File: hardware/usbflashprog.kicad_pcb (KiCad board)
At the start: 2 copper layers, 211 x 122 mm, 121 parts, among them J2 Parallel Adapter, J3 Serial Adapter, Q1 BC547, Q10 BC557, Q11 BC557, Q12 BC547, Q13 BC547, Q14 BC547, Q15 BC547, Q16 BC547, Q2 BC327, Q3 BC327, Q4 BC327, Q5 TIP120, Q6 BC327, Q7 BC557, Q8 BC557, Q9 BC557, U1 MT3608 Module, U10 74HC595, U11 74HC165, U12 74HC165, U2 74LS06N, U3 Pico, U4 74HC595, U5 74HC595, U6 74HC595, U7 74HC595, U8 74LS06N, U9 74HC595

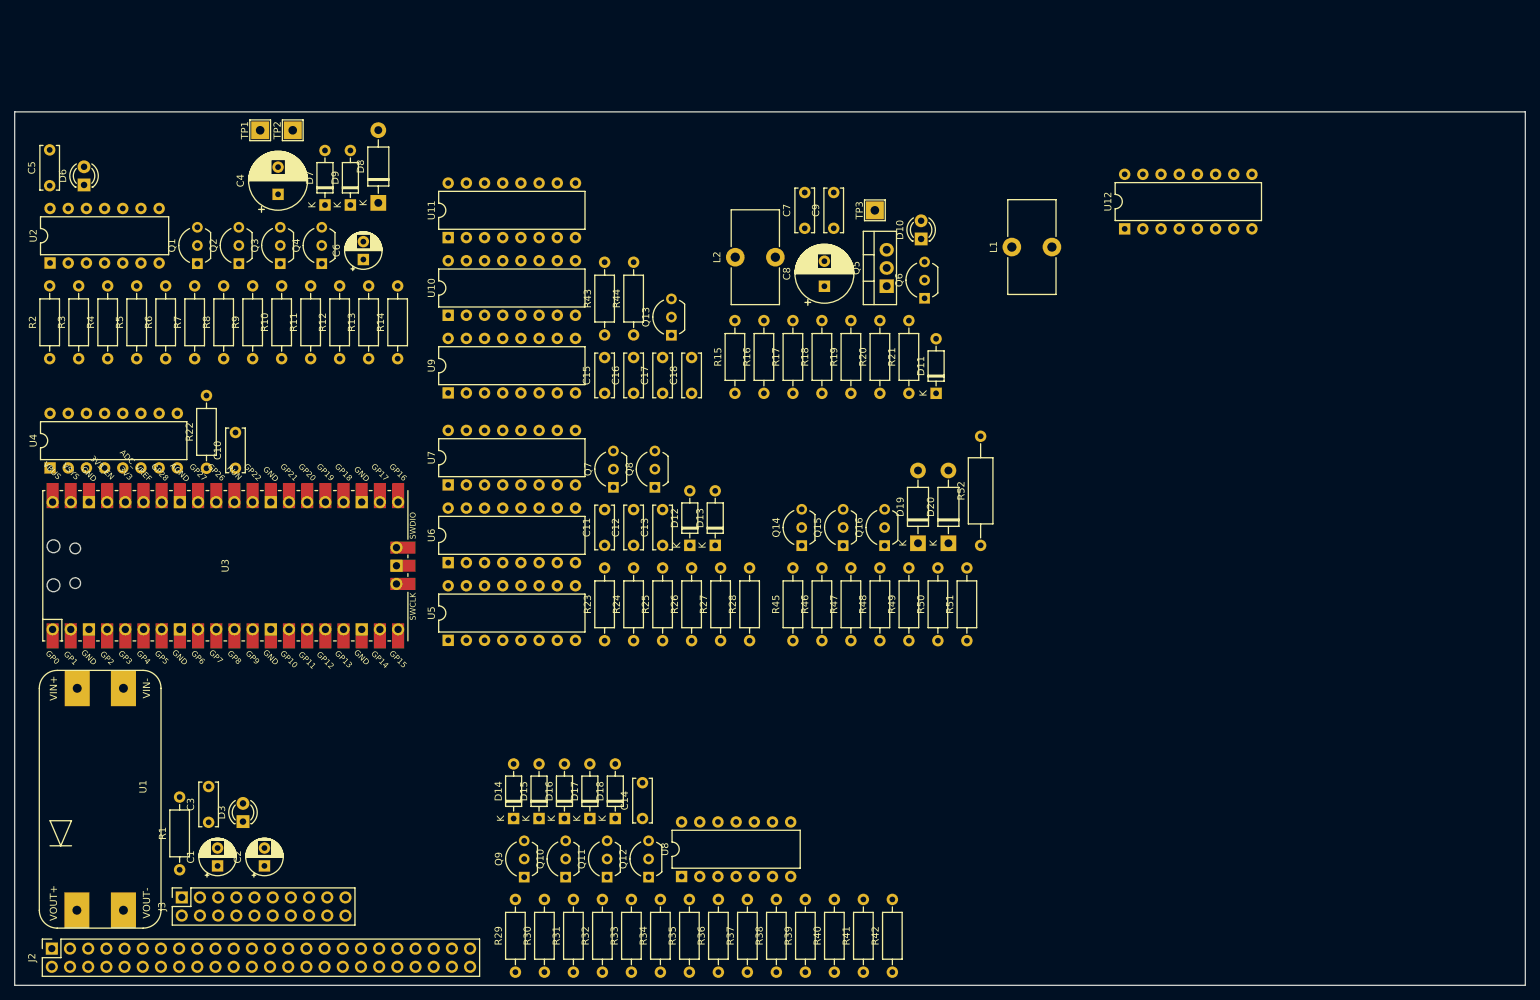
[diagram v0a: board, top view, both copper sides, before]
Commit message: 0.3.rev.A. Created new main pcb
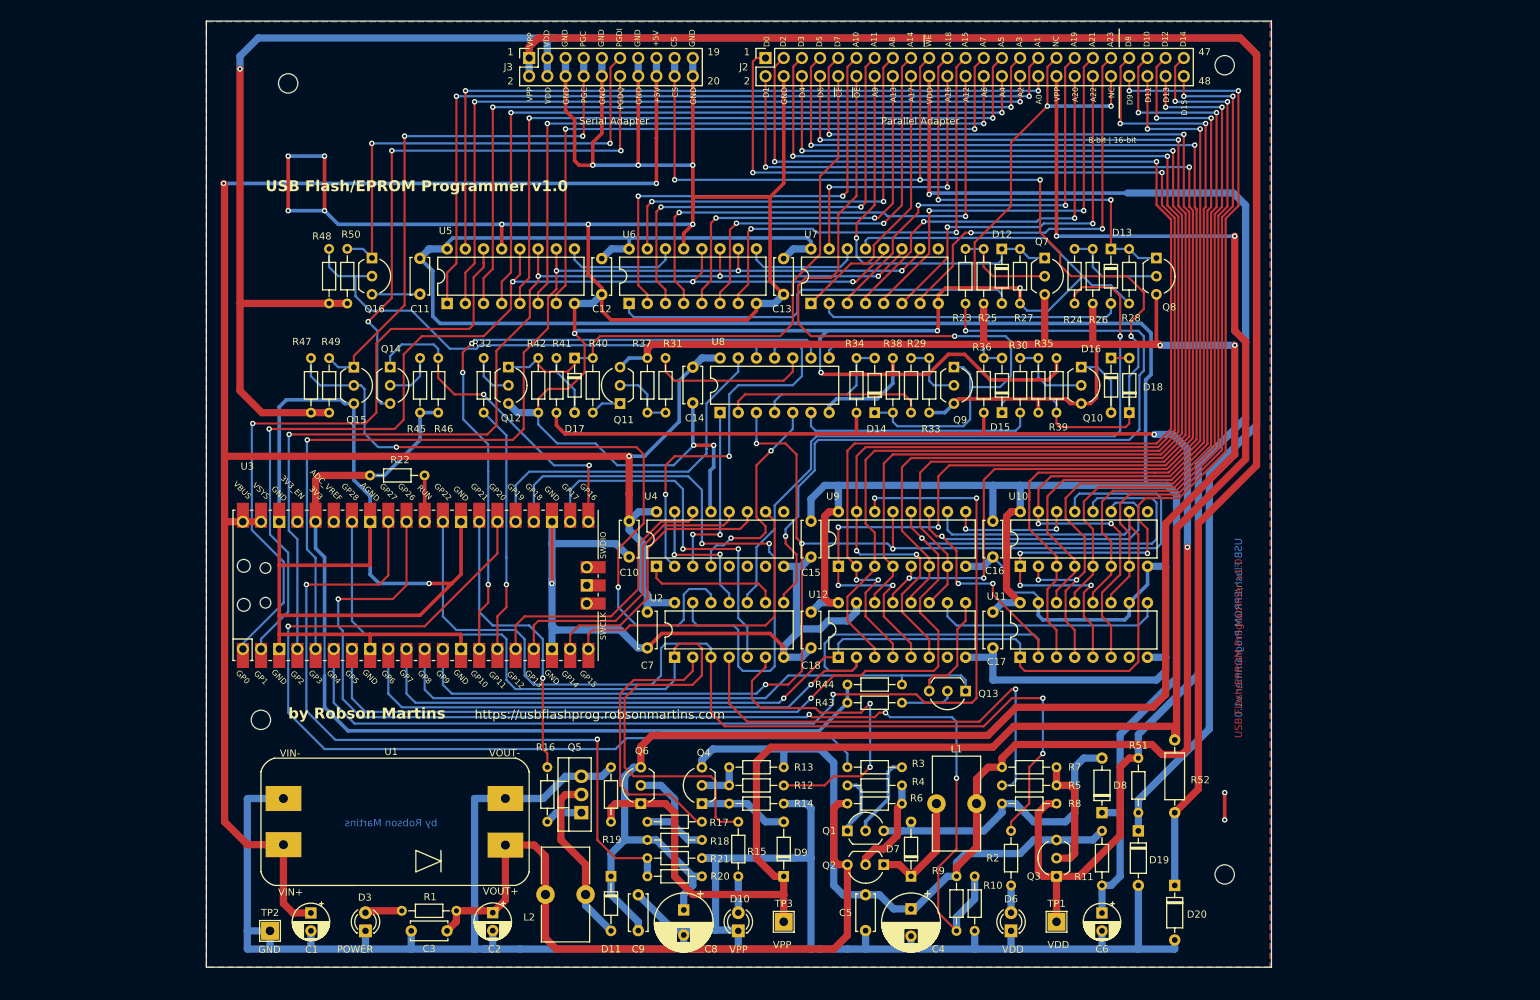
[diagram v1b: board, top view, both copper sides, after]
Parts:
- added ?: , , F.Cu at (72.4, 121.9)
- added ?: , , F.Cu at (207.0, 30.5)
- added ?: , , F.Cu at (207.0, 143.5)
- added REF**: MountingHole_2.7mm, MountingHole:MountingHole_2.7mm, F.Cu at (76.2, 33.0)
- C10, C11, C12, C13, C14, C15, C16, C17, C18, C3, C5, C7, C9: footprint Capacitor_THT:C_Disc_D6.0mm_W2.5mm_P5.00mm -> Capacitor_THT:C_Disc_D5.0mm_W2.5mm_P5.00mm
- D11, D12, D13, D14, D15, D16, D17, D18, D7, D9: footprint Diode_THT:D_DO-35_SOD27_P7.62mm_Horizontal -> Diode_THT:D_DO-34_SOD68_P7.62mm_Horizontal
- D19, D20, D8: footprint Diode_THT:D_DO-41_SOD81_P10.16mm_Horizontal -> Diode_THT:D_DO-35_SOD27_P7.62mm_Horizontal
- R1, R10, R11, R12, R13, R14, R15, R16, R17, R18, R19, R2, R20, R21, R22, R23, R24, R25, R26, R27, R28, R29, R3, R30, R31, R32, R33, R34, R35, R36, R37, R38, R39, R4, R40, R41, R42, R43, R44, R45, R46, R47, R48, R49, R5, R50, R51, R6, R7, R8, R9: footprint Resistor_THT:R_Axial_DIN0207_L6.3mm_D2.5mm_P10.16mm_Horizontal -> Resistor_THT:R_Axial_DIN0204_L3.6mm_D1.6mm_P7.62mm_Horizontal
- R52: footprint Resistor_THT:R_Axial_DIN0309_L9.0mm_D3.2mm_P15.24mm_Horizontal -> Resistor_THT:R_Axial_DIN0207_L6.3mm_D2.5mm_P10.16mm_Horizontal
- moved D6 166.2 mm to (177.2, 151.4)
- moved J2 159.4 mm to (142.9, 29.5)
- moved TP1 156.8 mm to (183.5, 150.1)
- moved C5 151.0 mm to (156.8, 146.4), turned to -90 degrees
- moved R2 149.6 mm to (177.2, 137.4), turned to -90 degrees
- moved R5 141.6 mm to (183.5, 131.1), turned to 180 degrees
- moved Q3 138.1 mm to (183.5, 143.8)
- moved C6 137.7 mm to (189.9, 148.9), turned to -90 degrees
- moved C4 133.3 mm to (163.2, 148.3), turned to -90 degrees
- moved R11 132.8 mm to (189.9, 145.0)
- moved D8 132.2 mm to (189.9, 134.9)
- moved R8 131.9 mm to (183.5, 133.6), turned to 180 degrees
- moved R3 128.4 mm to (161.9, 128.5), turned to 180 degrees
- moved J3 126.9 mm to (109.9, 29.5)
- moved R7 126.4 mm to (175.9, 128.5), turned to 0 degrees
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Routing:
- net GND: track 0.00 -> 1293.8 mm, vias 0 -> 22
- net VCC: track 0.00 -> 373.1 mm
- net VDD5: track 0.00 -> 341.3 mm, vias 0 -> 1
- net VPP_RAW: track 0.00 -> 324.9 mm, vias 0 -> 2
- net +5V: track 0.00 -> 307.4 mm, vias 0 -> 3
- net VDD_RAW: track 0.00 -> 271.8 mm, vias 0 -> 2
- net VPP: track 0.00 -> 246.1 mm, vias 0 -> 2
- net VPP13: track 0.00 -> 228.0 mm
- net /D1: track 0.00 -> 196.7 mm, vias 0 -> 6
- net /D0: track 0.00 -> 196.3 mm, vias 0 -> 4
- net VDD: track 0.00 -> 190.0 mm, vias 0 -> 1
- net /D2: track 0.00 -> 187.7 mm, vias 0 -> 4
- net /CPU/DCLK: track 0.00 -> 184.8 mm, vias 0 -> 4
- net /D3: track 0.00 -> 182.3 mm, vias 0 -> 2
- net /CPU/OE: track 0.00 -> 174.9 mm, vias 0 -> 4
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- added copper zone on B.Cu, net GND
- added copper zone on F.Cu, net GND
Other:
- board size 211 x 122 mm -> 148.8 x 132.2 mm
- board text added: "+5V"
- board text added: "1"
- board text added: "19"
- board text added: "2"
- board text added: "20"
- board text added: "47"
- board text added: "48"
- board text added: "8-bit | 16-bit"
- board text added: "A0"
- board text added: "A1"
- board text added: "A10"
- board text added: "A11"
- board text added: "A12"
- board text added: "A13"
- board text added: "A14"
- board text added: "A15"
- board text added: "A16"
- board text added: "A17"
- board text added: "A18"
- board text added: "A19"
- board text added: "A2"
- board text added: "A20"
- board text added: "A21"
- board text added: "A22"
- board text added: "A23"
- board text added: "A3"
- board text added: "A4"
- board text added: "A5"
- board text added: "A6"
- board text added: "A7"
- board text added: "A8"
- board text added: "A9"
- board text added: "CS"
- board text added: "D0"
- board text added: "D1"
- board text added: "D10"
- board text added: "D11"
- board text added: "D12"
- board text added: "D13"
- board text added: "D14"
- board text added: "D15"
- board text added: "D2"
- board text added: "D3"
- board text added: "D4"
- board text added: "D5"
- board text added: "D6"
- board text added: "D7"
- board text added: "D8"
- board text added: "D9"
- board text added: "GND"
- board text added: "NC"
- board text added: "PGC"
- board text added: "PGDI"
- board text added: "PGDQ"
- board text added: "POWER"
- board text added: "Parallel Adapter"
- board text added: "Serial Adapter"
- board text added: "USB Flash/EPROM Programmer v1.0"
- board text added: "VDD"
- board text added: "VPP"
- board text added: "by Robson Martins"
- board text added: "https://usbflashprog.robsonmartins.com"
- board text added: "~{CE}"
- board text added: "~{OE}"
- board text added: "~{WE}"
